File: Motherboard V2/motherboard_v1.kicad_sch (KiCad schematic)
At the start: 74 parts, among them J10 Conn_01x02, J11 Conn_01x02, J12 Conn_01x03_Pin, J13 Conn_01x03_Pin, J14 436500427, J15 Conn_01x01, J16 Conn_01x01, J17 Conn_01x02, J18 Conn_01x02, U1 PhotoMos, q10 Conn_01x07, q4 Conn_01x07, q5 Conn_01x07, q6 Conn_01x07, q8 Conn_01x07, q9 Conn_01x07

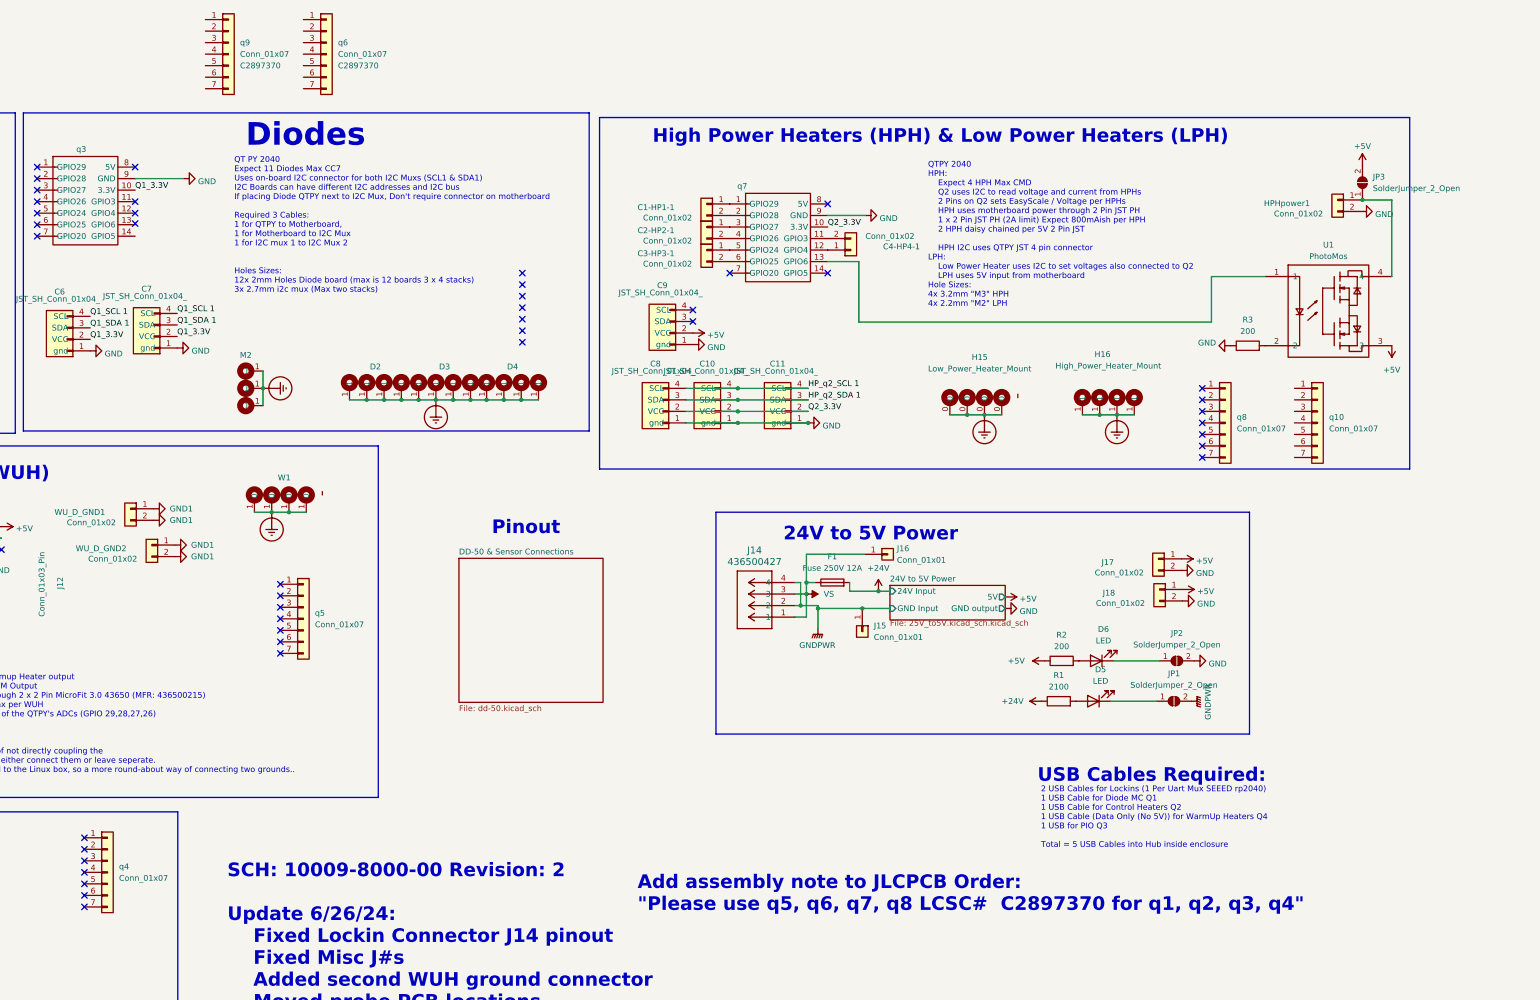
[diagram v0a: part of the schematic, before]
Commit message: update
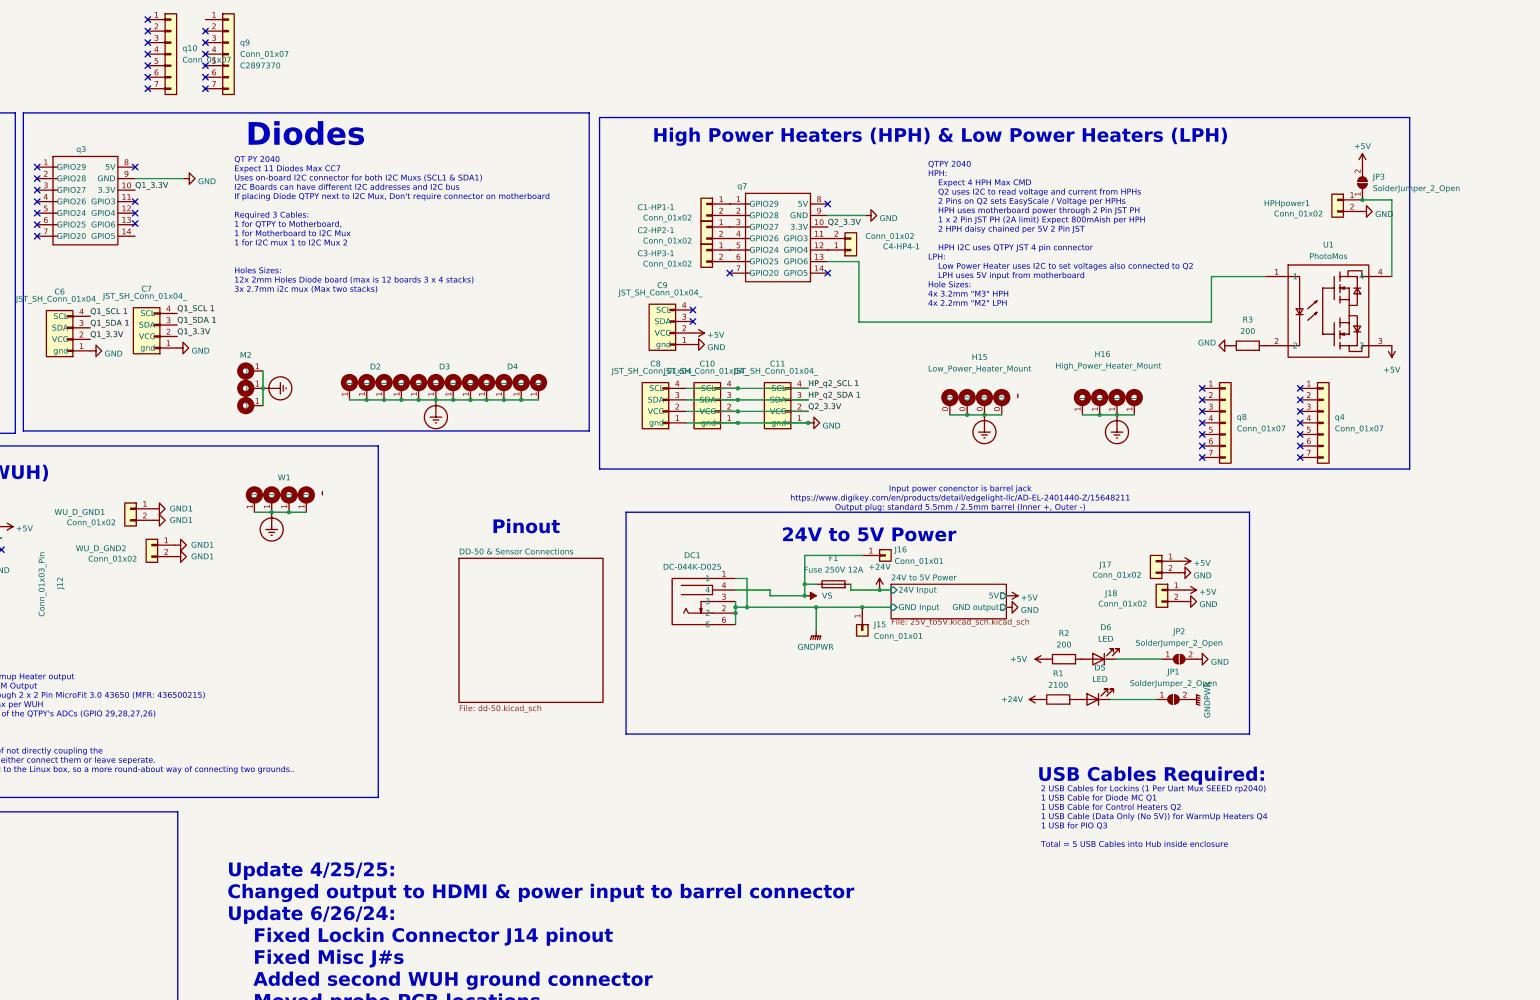
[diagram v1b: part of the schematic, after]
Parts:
- removed J14: 436500427, 0_Motherboard_v1:CON_436500427_MOL, symbol 0_mb_library:436500427
- removed q5, q6: Conn_01x07, Connector_PinSocket_2.54mm:PinSocket_1x07_P2.54mm_Vertical, symbol Connector_Generic:Conn_01x07
- added DC1: DC-044K-D025, 0_Motherboard_v1:barrel_jack_DC-IN-TH_DC-044K-D025, symbol 0_mb_library:DC-044K-D025
- q1, q2, q3, q7: LCSC C2897370 -> (none)
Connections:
- net GNDPWR: now also DC1.1, DC1.2, DC1.3, DC1.6
- net VS: now also DC1.4
- no-connect marks 59 -> 58
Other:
- note added: "Input power conenctor is barrel jack https://www.digikey.com/en/products/detail/edgelight-llc/AD-EL-2401440-Z/15648211 Output plug: standard 5.5mm / 2.5mm barrel (Inner +, Outer -)"
- note added: "Update 4/25/25: Changed output to HDMI & power input to barrel connector Update 6/26/24: Fixed Lockin Connector J14 pinout Fixed Misc J#s Added second WUH ground connector Moved probe PCB locations Added silkscreen rev # Update 5/14/24: Fixed 50 dsub pinout Fixed 50 dsub mounting hole diameter Changed modular circuit holes to M3 Clearance. Added more 24V grounding vias Added WUH grounding cable a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"
- note removed: "Add assembly note to JLCPCB Order: "Please use q5, q6, q7, q8 LCSC# C2897370 for q1, q2, q3, q4""
- note removed: "SCH: 10009-8000-00 Revision: 2 Update 6/26/24: Fixed Lockin Connector J14 pinout Fixed Misc J#s Added second WUH ground connector Moved probe PCB locations Added silkscreen rev # Update 5/14/24: Fixed 50 dsub pinout Fixed 50 dsub mounting hole diameter Changed modular circuit holes to M3 Clearance. Added more 24V grounding vias Added WUH grounding cable and ability to not directly couple 24V gnd 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"
- moved on the sheet: D6, J16, J17, J18, JP2, R2, q10, q4
